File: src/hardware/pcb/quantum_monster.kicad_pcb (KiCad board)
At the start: 2 copper layers, 51.9 x 39.9 mm, 28 parts, among them J1 ICSP, J2 PCD8544, Q1 VS1838B, SW1 RESET, SW2 A, SW3 B, SW4 C, U1 ATmega328P-PU, Y1 32.768kHz

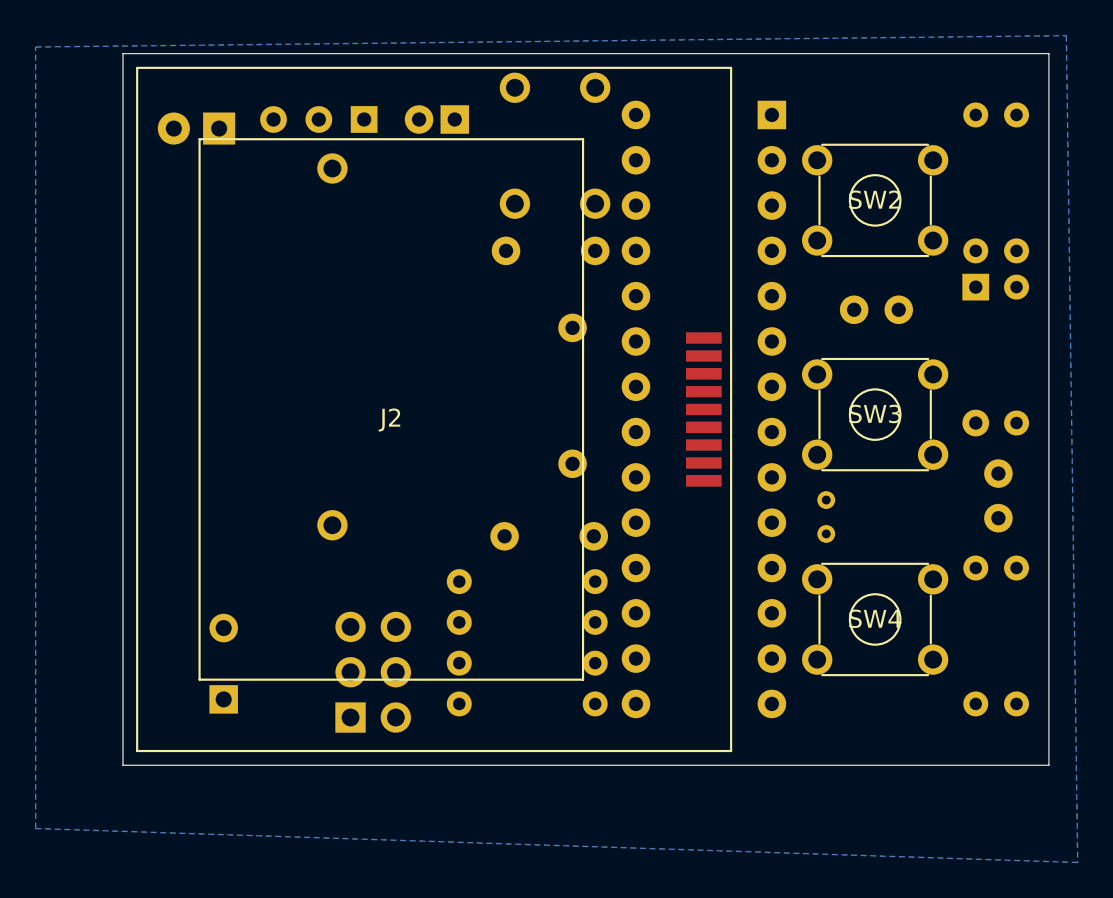
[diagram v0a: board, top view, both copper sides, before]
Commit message: Initial production prototype of PCB.
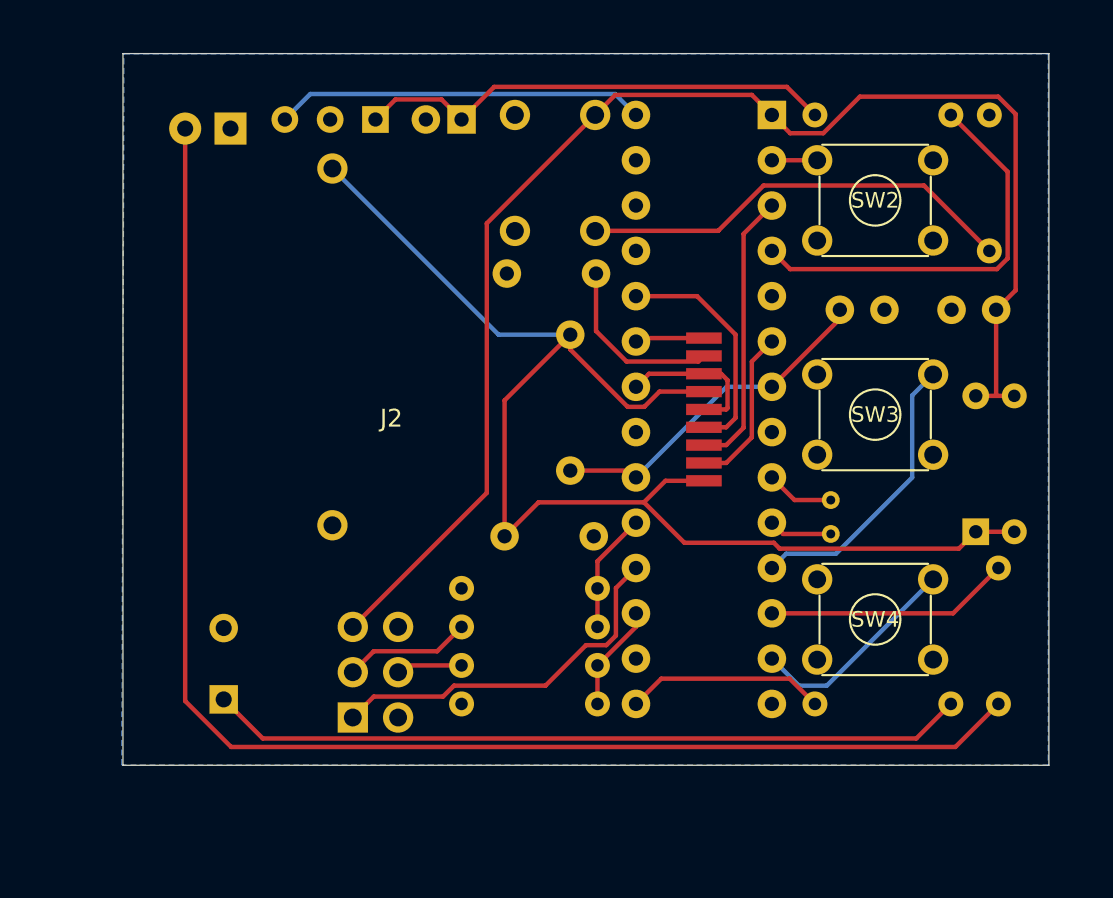
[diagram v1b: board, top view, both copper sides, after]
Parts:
- moved D1 13.7 mm to (138.4, 102.1), turned to 90 degrees
- moved SW1 9.20 mm to (117.1, 85.2), turned to 90 degrees
- moved C1 9.18 mm to (139.6, 89.7), turned to 180 degrees
- moved R9 9.02 mm to (129.4, 78.7), turned to 0 degrees
- moved R3 8.81 mm to (117.2, 105.3), turned to 180 degrees
- moved R7 7.75 mm to (137.0, 111.8), turned to 180 degrees
- moved R8 7.69 mm to (139.7, 111.8), turned to 90 degrees
- moved R6 6.86 mm to (117.2, 111.8)
- moved R1 6.10 mm to (140.6, 94.5)
- moved R4 4.32 mm to (109.6, 107.4)
- moved R5 2.42 mm to (117.2, 109.6)
- moved R2 1.52 mm to (139.2, 78.7)
- moved C4 1.27 mm to (117.1, 87.6)
- moved C2 0.80 mm to (130.8, 89.7)
- moved D2 0.64 mm to (96.6, 79.5)
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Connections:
- net DISPLAY_CLOCK renamed DISPLAY_SCLK
- net DISPLAY_MOSI renamed DISPLAY_SDIN
- J1 pad 2: Net-(J1-Pad2) -> unconnected-(J1-Pad2)
- J2 pad 1: DISPLAY_RESET -> DISPLAY_RES
- J2 pad 6: DISPLAY_DATA_COMMAND -> DISPLAY_DC
- Q1 pad 3: LINK_RECEIVER_DATA -> INFRARED_RECEIVER_OUT
- R8 pad 2: LINK_TRANSMITTER -> INFRARED_TRANSMITTER
- R9 pad 2: LINK_RECEIVER_POWER -> INFRARED_RECEIVER_POWER
- SW2 pad 1: GND -> A_BUTTON
- SW2 pad 2: A_BUTTON -> GND
- U1 pad 11: DISPLAY_DATA_COMMAND -> B_BUTTON
- U1 pad 12: SPEAKER -> INFRARED_TRANSMITTER
- U1 pad 13: Net-(U1-Pad13) -> C_BUTTON
- U1 pad 14: Net-(U1-Pad14) -> unconnected-(U1-Pad14)
- U1 pad 15: LINK_TRANSMITTER -> SPEAKER
- U1 pad 16: Net-(U1-Pad16) -> unconnected-(U1-Pad16)
- U1 pad 2: Net-(U1-Pad2) -> A_BUTTON
- U1 pad 21: Net-(U1-Pad21) -> unconnected-(U1-Pad21)
- U1 pad 23: Net-(U1-Pad23) -> DISPLAY_RES
- U1 pad 24: DISPLAY_RESET -> DISPLAY_DC
- U1 pad 25: C_BUTTON -> unconnected-(U1-Pad25)
- U1 pad 26: Net-(U1-Pad26) -> unconnected-(U1-Pad26)
- U1 pad 27: LINK_RECEIVER_DATA -> unconnected-(U1-Pad27)
- U1 pad 28: LINK_RECEIVER_POWER -> INFRARED_RECEIVER_OUT
- U1 pad 4: Net-(U1-Pad4) -> INFRARED_RECEIVER_POWER
- U1 pad 5: Net-(U1-Pad5) -> unconnected-(U1-Pad5)
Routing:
- net Net-(D2-Pad2): track 0.00 -> 79.8 mm
- net RESET: track 0.00 -> 78.9 mm
- net VCC: track 0.00 -> 74.7 mm
- net Net-(BZ1-Pad1): track 0.00 -> 42.5 mm
- net Net-(C5-Pad1): track 0.00 -> 27.0 mm
- net Net-(R2-Pad2): track 0.00 -> 24.7 mm
- net INFRARED_RECEIVER_POWER: track 0.00 -> 23.3 mm
- net MISO: track 0.00 -> 20.9 mm
- net INFRARED_RECEIVER_OUT: track 0.00 -> 20.8 mm
- net FILTERED_VCC: track 0.00 -> 19.5 mm
- net B_BUTTON: track 0.00 -> 16.2 mm
- net DISPLAY_SDIN: track 0.00 -> 15.7 mm
- net INFRARED_TRANSMITTER: track 0.00 -> 13.8 mm
- net DISPLAY_DC: track 0.00 -> 13.1 mm
- net C_BUTTON: track 0.00 -> 12.1 mm
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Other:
- board text added: "GND"
- board text added: "MISO"
- board text added: "MOSI"
- board text added: "NC"
- board text added: "RST"
- board text added: "SCK"
